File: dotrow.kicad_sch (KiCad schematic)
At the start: 48 parts, among them J1 Conn_01x02_Pin, J2 Conn_01x02_Pin, J3 Conn_01x02_Pin, J4 Conn_01x12_Pin, U5 74HC595

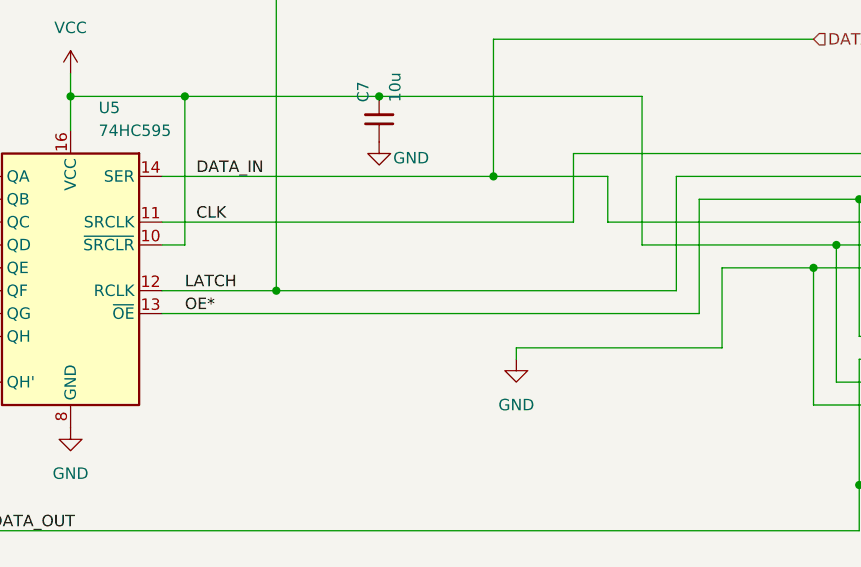
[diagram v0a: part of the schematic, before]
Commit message: valid 13 row layout
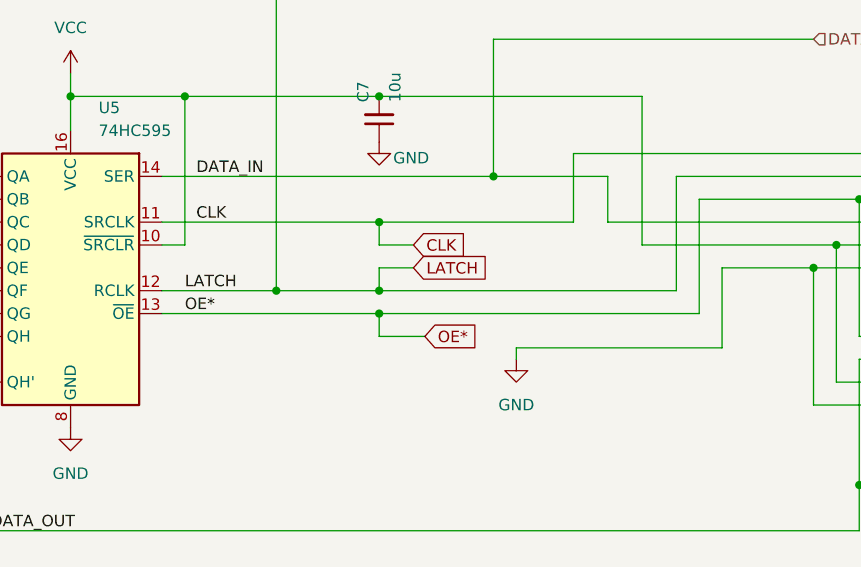
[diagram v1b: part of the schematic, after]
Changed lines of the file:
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@@
 	(paper "A4")
 	(junction
+		(at 179.07 86.36)
+		(diameter 0)
+		(color 0 0 0 0)
+	)
+	(junction
 		(at 191.77 73.66)
 		(diameter 0)
@@
 	)
 	(junction
+		(at 179.07 88.9)
+		(diameter 0)
+		(color 0 0 0 0)
+	)
+	(junction
 		(at 50.8 29.21)
 		(diameter 0)
@@
 	(junction
 		(at 69.85 26.67)
+		(diameter 0)
+		(color 0 0 0 0)
+	)
+	(junction
+		(at 179.07 78.74)
 		(diameter 0)
 		(color 0 0 0 0)
@@
 	(wire
 		(pts
+			(xy 179.07 86.36) (xy 212.09 86.36)
+		)
+		(stroke
+			(width 0)
+			(type default)
+		)
+	)
+	(wire
+		(pts
 			(xy 74.93 41.91) (xy 69.85 41.91)
 		)
@@
 	(wire
 		(pts
-			(xy 154.94 88.9) (xy 214.63 88.9)
+			(xy 154.94 88.9) (xy 179.07 88.9)
 		)
 		(stroke
@@
 	(wire
 		(pts
+			(xy 179.07 91.44) (xy 179.07 88.9)
+		)
+		(stroke
+			(width 0)
+			(type default)
+		)
+	)
+	(wire
+		(pts
 			(xy 234.95 73.66) (xy 240.03 73.66)
 		)
@@
 	(wire
 		(pts
+			(xy 179.07 78.74) (xy 200.66 78.74)
+		)
+		(stroke
+			(width 0)
+			(type default)
+		)
+	)
+	(wire
+		(pts
 			(xy 92.71 149.86) (xy 106.68 149.86)
 		)
@@
 	(wire
 		(pts
-			(xy 167.64 86.36) (xy 212.09 86.36)
+			(xy 167.64 86.36) (xy 179.07 86.36)
 		)
 		(stroke
@@
 	(wire
 		(pts
+			(xy 179.07 83.82) (xy 179.07 86.36)
+		)
+		(stroke
+			(width 0)
+			(type default)
+		)
+	)
+	(wire
+		(pts
 			(xy 40.64 129.54) (xy 40.64 133.35)
 		)
@@
 	(wire
 		(pts
+			(xy 179.07 88.9) (xy 214.63 88.9)
+		)
+		(stroke
+			(width 0)
+			(type default)
+		)
+	)
+	(wire
+		(pts
 			(xy 45.72 29.21) (xy 50.8 29.21)
 		)
@@
 	(wire
 		(pts
+			(xy 182.88 83.82) (xy 179.07 83.82)
+		)
+		(stroke
+			(width 0)
+			(type default)
+		)
+	)
+	(wire
+		(pts
 			(xy 144.78 64.77) (xy 144.78 68.58)
 		)
@@
 	(wire
 		(pts
+			(xy 182.88 81.28) (xy 179.07 81.28)
+		)
+		(stroke
+			(width 0)
+			(type default)
+		)
+	)
+	(wire
+		(pts
 			(xy 50.8 114.3) (xy 74.93 114.3)
 		)
@@
 	(wire
 		(pts
+			(xy 184.15 91.44) (xy 179.07 91.44)
+		)
+		(stroke
+			(width 0)
+			(type default)
+		)
+	)
+	(wire
+		(pts
 			(xy 69.85 41.91) (xy 69.85 39.37)
 		)
@@
 	(wire
 		(pts
+			(xy 179.07 81.28) (xy 179.07 78.74)
+		)
+		(stroke
+			(width 0)
+			(type default)
+		)
+	)
+	(wire
+		(pts
 			(xy 232.41 113.03) (xy 232.41 107.95)
 		)
@@
 	(wire
 		(pts
-			(xy 154.94 78.74) (xy 200.66 78.74)
+			(xy 154.94 78.74) (xy 179.07 78.74)
 		)
 		(stroke
@@
 		)
 	)
+	(global_label "LATCH"
+		(shape input)
+		(at 182.88 83.82 0)
+		(fields_autoplaced yes)
+		(effects
+			(font
+				(size 1.27 1.27)
+			)
+			(justify left)
+		)
+		(property "Intersheetrefs" "${INTERSHEET_REFS}"
+			(at 191.55 83.82 0)
+			(effects
+				(font
+					(size 1.27 1.27)
+				)
+				(justify left)
+				(hide yes)
+			)
+		)
+	)
+	(global_label "CLK"
+		(shape input)
+		(at 182.88 81.28 0)
+		(fields_autoplaced yes)
+		(effects
+			(font
+				(size 1.27 1.27)
+			)
+			(justify left)
+		)
+		(property "Intersheetrefs" "${INTERSHEET_REFS}"
+			(at 189.4333 81.28 0)
+			(effects
+				(font
+					(size 1.27 1.27)
+				)
+				(justify left)
+				(hide yes)
+			)
+		)
+	)
+	(global_label "OE*"
+		(shape input)
+		(at 184.15 91.44 0)
+		(fields_autoplaced yes)
+		(effects
+			(font
+				(size 1.27 1.27)
+			)
+			(justify left)
+		)
+		(property "Intersheetrefs" "${INTERSHEET_REFS}"
+			(at 190.5823 91.44 0)
+			(effects
+				(font
+					(size 1.27 1.27)
+				)
+				(justify left)
+				(hide yes)
+			)
+		)
+	)
